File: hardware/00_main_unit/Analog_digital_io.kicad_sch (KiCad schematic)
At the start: 4 parts, among them IC3 74HC14D

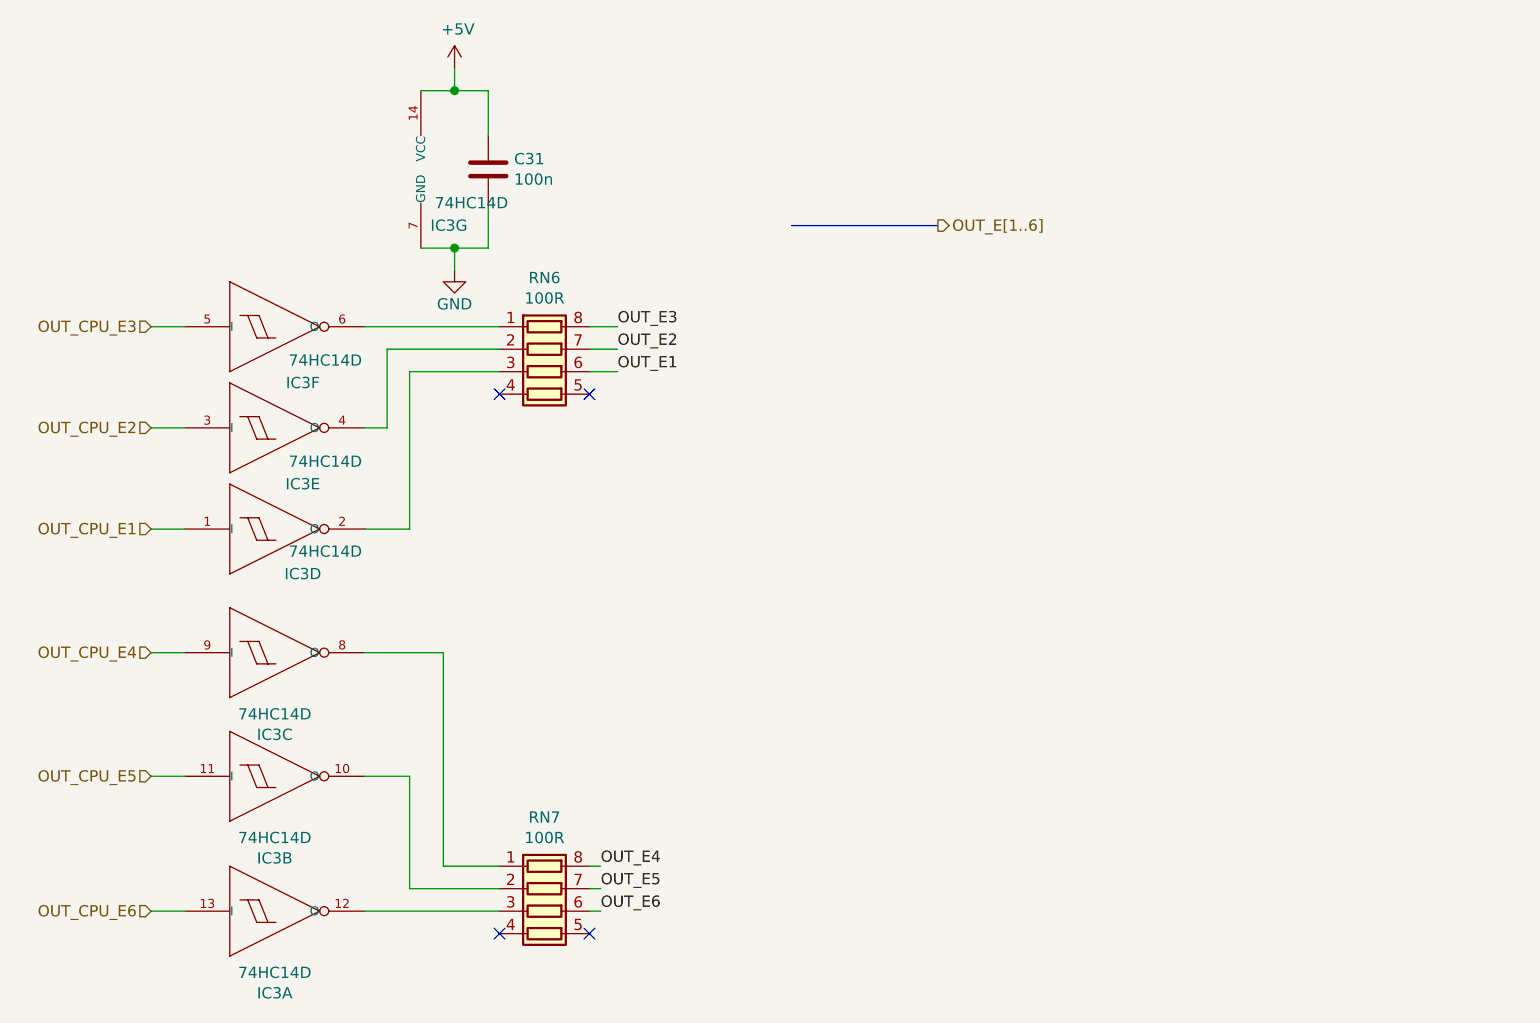
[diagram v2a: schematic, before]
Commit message: FW and SW updates for new revision
Signed-off-by: Jarosław Karwik <jaroslaw.karwik@gmail.com>
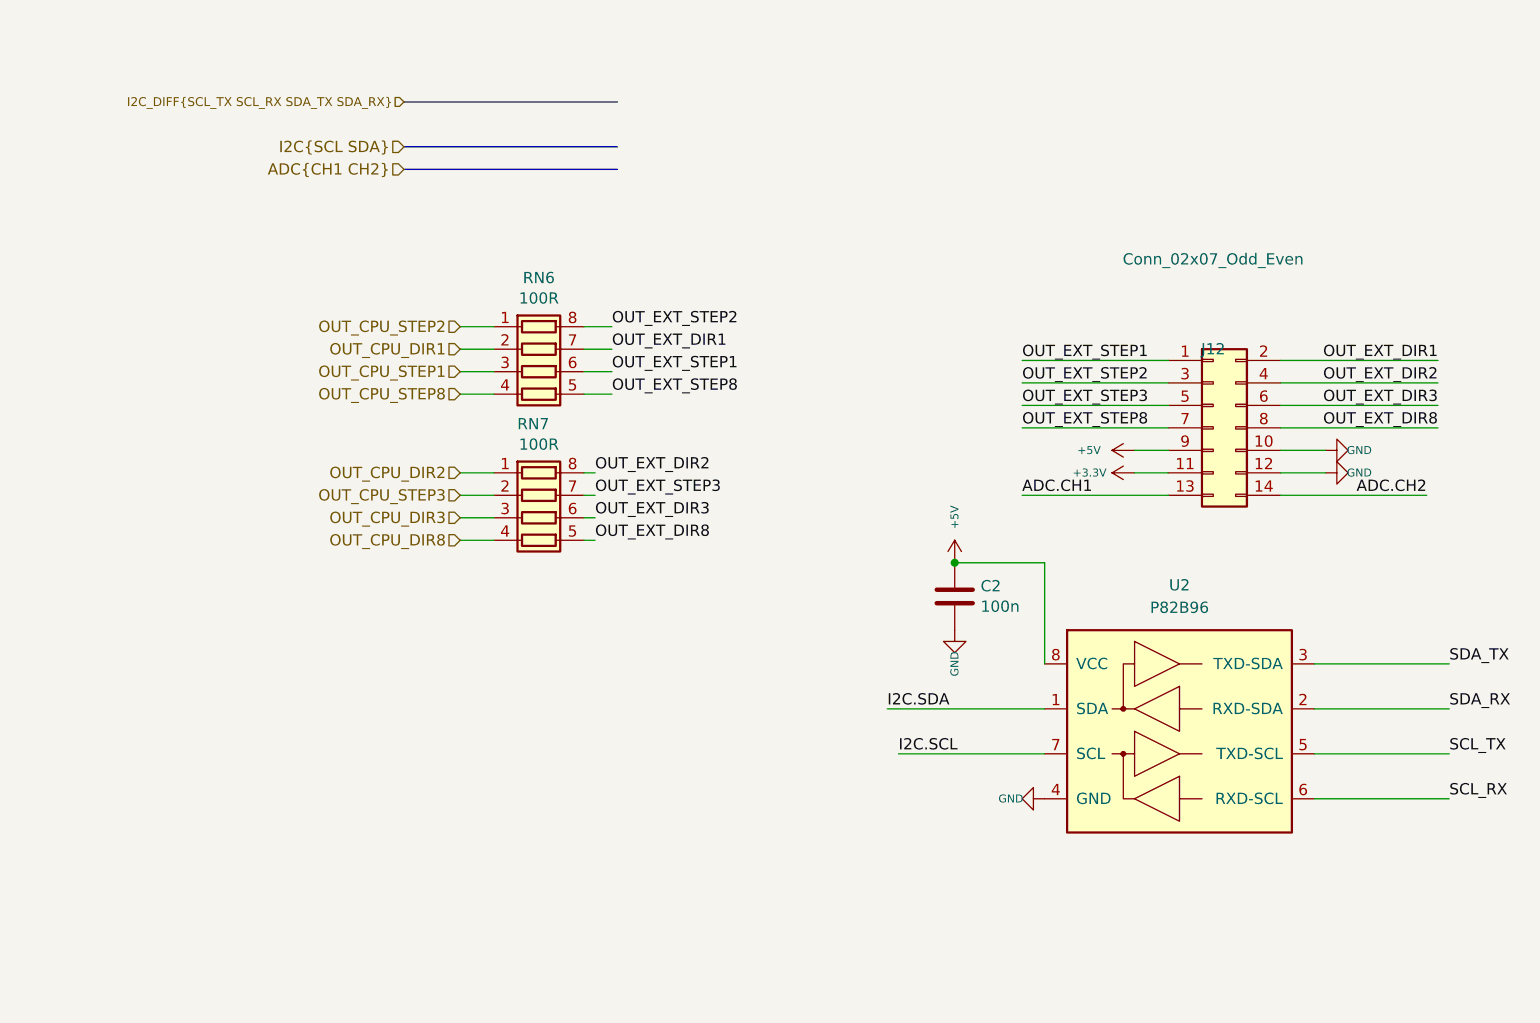
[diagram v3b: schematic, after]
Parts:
- removed C31: 100n, Capacitor_SMD:C_0603_1608Metric, symbol Uni_Printer-rescue:C-Device
- removed IC3: 74HC14D, moje:SO14, symbol Uni_Printer-rescue:74*14-step2cnc-Uni_Printer_v1-rescue
- added C2: 100n, Capacitor_SMD:C_0603_1608Metric, symbol Uni_Printer-rescue:C-Device
- added J12: Conn_02x07_Odd_Even, Connector_PinHeader_2.54mm:PinHeader_2x07_P2.54mm_Vertical, symbol Connector_Generic:Conn_02x07_Odd_Even
- added U2: P82B96, Package_SO:TSSOP-8_4.4x3mm_P0.65mm, symbol Interface_Expansion:P82B96
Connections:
- net +5V: now also C2.1, J12.9 (Pin_9), U2.8 (VCC)
- net GND: now also C2.2, J12.10 (Pin_10), J12.12 (Pin_12), U2.4 (GND)
- net OUT_CPU_DIR2: now reaches RN7.1 (R1.1)
- net OUT_CPU_STEP3: now reaches RN7.2 (R2.1)
- net OUT_CPU_DIR3: now reaches RN7.3 (R3.1)
- net OUT_CPU_STEP1: now reaches RN6.3 (R3.1)
- net OUT_CPU_DIR1: now reaches RN6.2 (R2.1)
- net OUT_CPU_STEP2: now reaches RN6.1 (R1.1)
- net OUT_CPU_STEP8: now reaches RN6.4 (R4.1)
- net OUT_EXT_STEP8: now reaches RN6.5 (R4.2)
- net OUT_EXT_STEP8: now also J12.7 (Pin_7)
- net OUT_CPU_DIR8: now reaches RN7.4 (R4.1)
- net OUT_EXT_DIR8: now reaches RN7.5 (R4.2)
- net OUT_EXT_DIR8: now also J12.8 (Pin_8)
- net OUT_E1 renamed OUT_EXT_STEP1
- net OUT_EXT_STEP1: now also J12.1 (Pin_1)
- net OUT_E2 renamed OUT_EXT_DIR1
- net OUT_EXT_DIR1: now also J12.2 (Pin_2)
- net OUT_E3 renamed OUT_EXT_STEP2
- net OUT_EXT_STEP2: now also J12.3 (Pin_3)
- net OUT_E4 renamed OUT_EXT_DIR2
- net OUT_EXT_DIR2: now also J12.4 (Pin_4)
- net OUT_E5 renamed OUT_EXT_STEP3
- net OUT_EXT_STEP3: now also J12.5 (Pin_5)
- net OUT_E6 renamed OUT_EXT_DIR3
- net OUT_EXT_DIR3: now also J12.6 (Pin_6)
- new net +3V3: J12.11 (Pin_11)
- new net ADC.CH1: J12.13 (Pin_13)
- new net ADC.CH2: J12.14 (Pin_14)
- new net I2C.SCL: U2.7 (SCL)
- new net I2C.SDA: U2.1 (SDA)
- new net SCL_RX: U2.6 (RXD-SCL)
- new net SCL_TX: U2.5 (TXD-SCL)
- new net SDA_RX: U2.2 (RXD-SDA)
- new net SDA_TX: U2.3 (TXD-SDA)
- no-connect marks 4 -> 0
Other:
- moved on the sheet: RN6, RN7
